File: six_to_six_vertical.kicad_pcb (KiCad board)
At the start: 2 copper layers, 99.1 x 99.1 mm, 12 parts, among them J1 RF Conn, J10 bnc, J11 bnc, J12 bnc, J2 RF Conn, J3 RF Conn, J4 RF Conn, J5 RF Conn, J6 RF Conn, J7 bnc, J8 bnc, J9 bnc

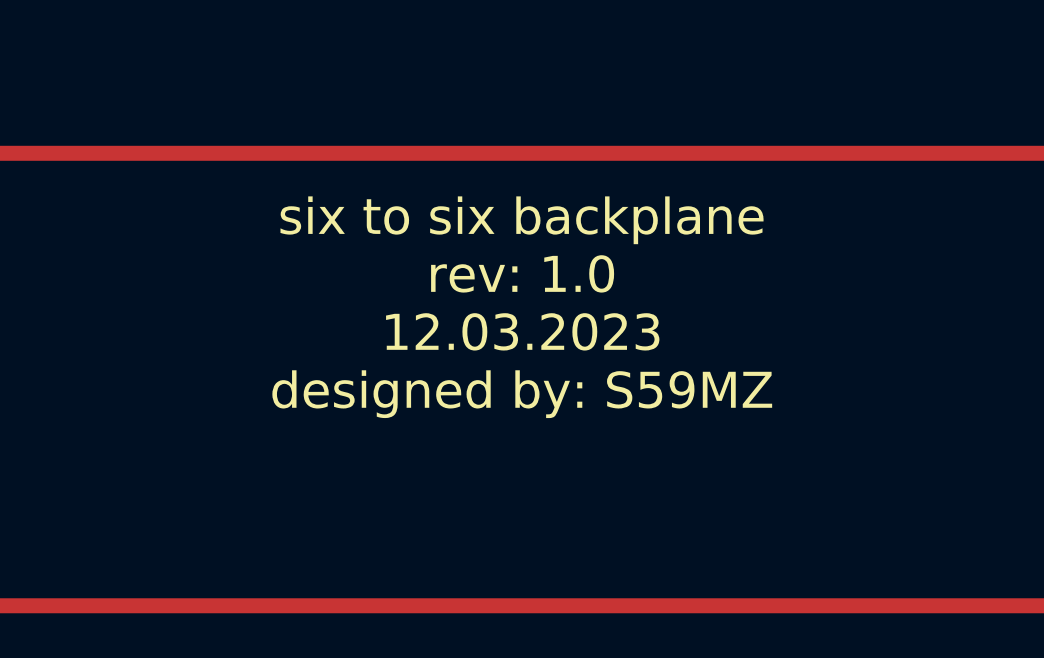
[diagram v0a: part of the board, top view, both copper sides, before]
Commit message: update board name
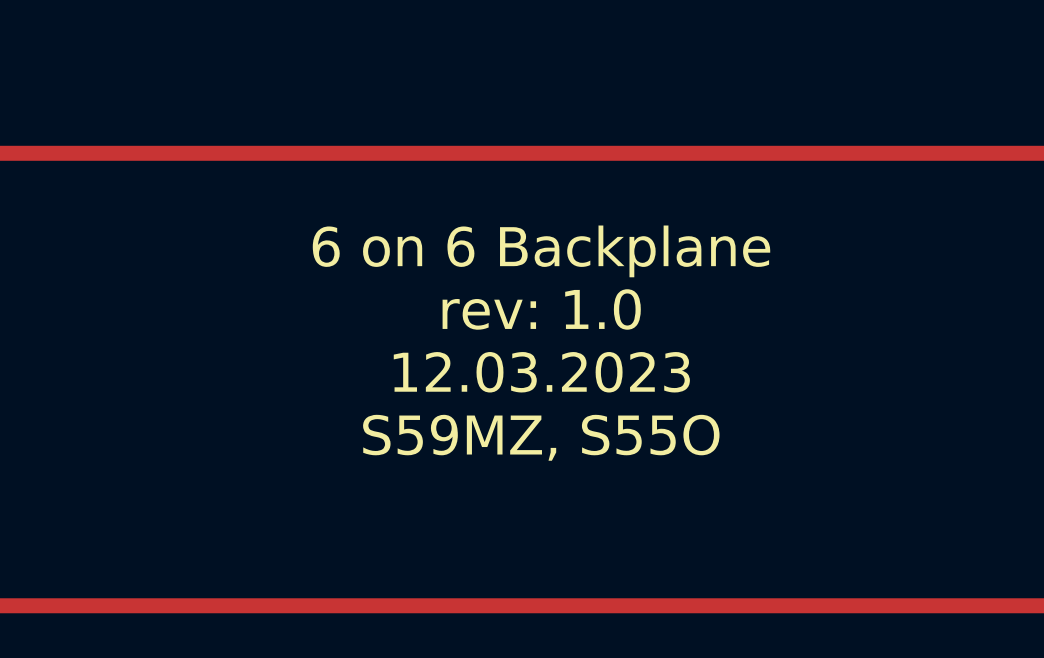
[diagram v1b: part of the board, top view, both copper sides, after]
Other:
- board text added: "6 on 6 Backplane rev: 1.0 12.03.2023 S59MZ, S55O"
- board text removed: "six to six backplane rev: 1.0 12.03.2023 designed by: S59MZ"
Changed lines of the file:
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@@
   (gr_arc locked (start 196.85 142.875) (mid 196.664013 143.324013) (end 196.215 143.51) (layer "Edge.Cuts") (width 0.1))
   (gr_line locked (start 97.79 45.085) (end 97.79 142.875) (layer "Edge.Cuts") (width 0.1))
-  (gr_text "six to six backplane\nrev: 1.0\n12.03.2023\ndesigned by: S59MZ" (at 147.955 63.5) (layer "F.SilkS")
-    (effects (font (size 1.2 1.2) (thickness 0.15)))
+  (gr_text "6 on 6 Backplane\nrev: 1.0\n12.03.2023\nS59MZ, S55O" (at 148.59 64.77) (layer "F.SilkS")
+    (effects (font (size 1.3 1.3) (thickness 0.15)))
   )
   (segment (start 176.8176 101.6) (end 178.9422 101.6) (width 0.5) (layer "F.Cu") (net 1))
